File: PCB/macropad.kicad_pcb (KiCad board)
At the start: 2 copper layers, 4 parts, among them SW1 SW_Push, SW2 SW_Push, SW3 SW_Push, U1 MOUDLE-SEEEDUINO-XIAO

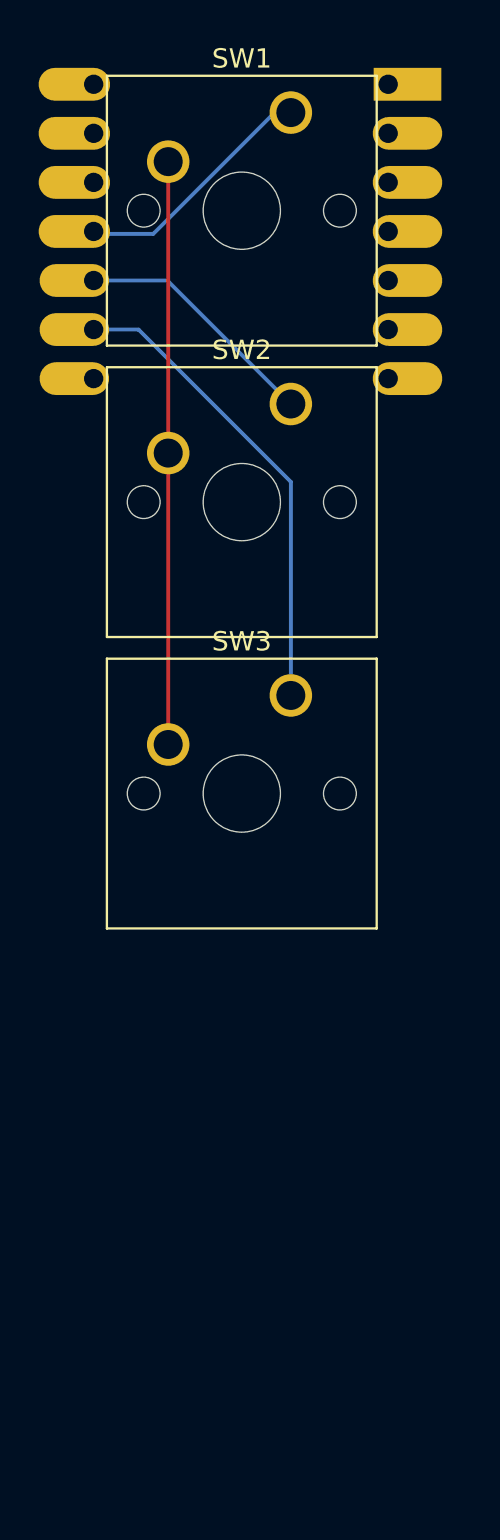
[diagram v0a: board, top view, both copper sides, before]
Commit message: Refactor code structure for improved readability and maintainability
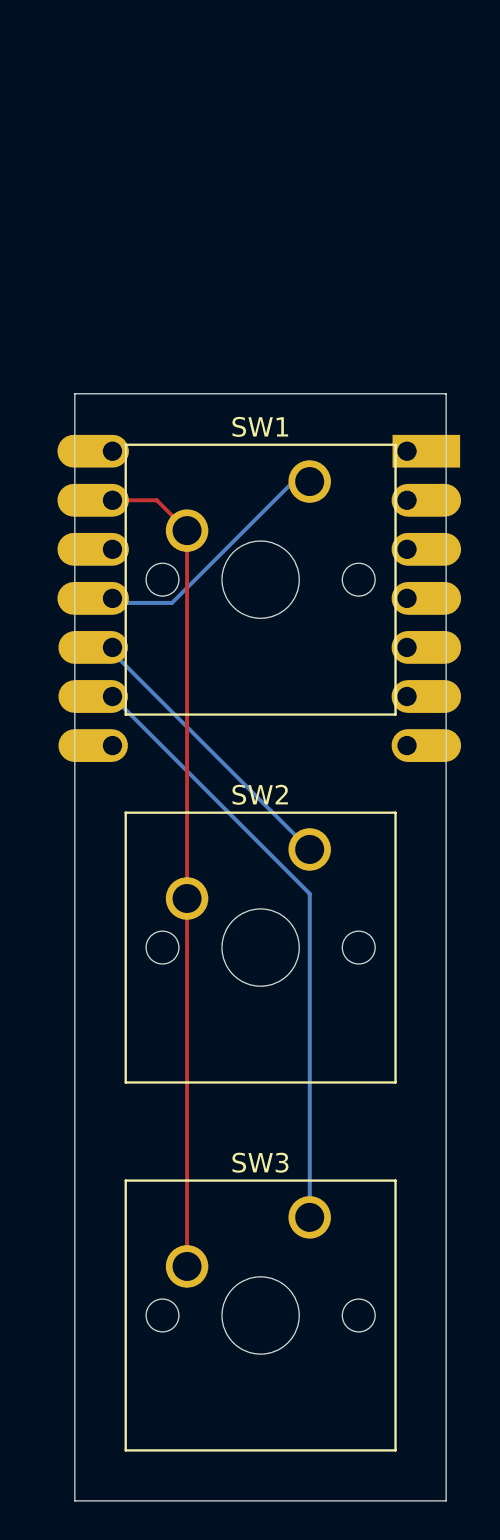
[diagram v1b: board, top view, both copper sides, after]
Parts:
- moved SW3 27.0 mm to (134.1, 119.2)
- moved SW2 23.1 mm to (134.1, 100.1)
- moved SW1 19.1 mm to (134.1, 81.1)
- moved U1 19.0 mm to (131.5, 87.1)
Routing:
- net GND: track 30.2 -> 42.7 mm
- net Net-(U1-PA7_A8_D8_SCK): track 24.5 -> 31.2 mm
- net Net-(U1-PA5_A9_D9_MISO): track 12.9 -> 14.7 mm
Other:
- board outline added: 19.2 x 57.3 mm
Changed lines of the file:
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@@
 	(footprint "Button_Switch_Keyboard:SW_Cherry_MX_1.00u_PCB"
 		(layer "F.Cu")
-		(at 133.085 61.965)
+		(at 134.06 81.07)
 		(descr "Cherry MX keyswitch, 1.00u, PCB mount, http://cherryamericas.com/wp-content/uploads/2014/12/mx_cat.pdf")
 		(tags "Cherry MX keyswitch 1.00u PCB")
@@
 	(footprint "Button_Switch_Keyboard:SW_Cherry_MX_1.00u_PCB"
 		(layer "F.Cu")
-		(at 133.085 77.055)
+		(at 134.06 100.12)
 		(descr "Cherry MX keyswitch, 1.00u, PCB mount, http://cherryamericas.com/wp-content/uploads/2014/12/mx_cat.pdf")
 		(tags "Cherry MX keyswitch 1.00u PCB")
@@
 	(footprint "Button_Switch_Keyboard:SW_Cherry_MX_1.00u_PCB"
 		(layer "F.Cu")
-		(at 133.085 92.145)
+		(at 134.06 119.17)
 		(descr "Cherry MX keyswitch, 1.00u, PCB mount, http://cherryamericas.com/wp-content/uploads/2014/12/mx_cat.pdf")
 		(tags "Cherry MX keyswitch 1.00u PCB")
@@
 	(footprint "footprints:XIAO-Generic-Hybrid-14P-2.54-21X17.8MM"
 		(layer "B.Cu")
-		(at 130.5 68.12 180)
+		(at 131.475 87.12 180)
 		(property "Reference" "U1"
 			(at 0 -2.54 0)
@@
 		(embedded_fonts no)
 	)
-	(segment
-		(start 126.735 94.685)
-		(end 126.735 79.595)
-		(width 0.2)
-		(layer "F.Cu")
-		(net "GND")
+	(gr_rect
+		(start 121.9 76.525)
+		(end 141.125 133.85)
+		(stroke
+			(width 0.05)
+			(type default)
+		)
+		(fill no)
+		(layer "Edge.Cuts")
 	)
 	(segment
-		(start 126.735 79.595)
-		(end 126.735 64.505)
+		(start 126.937056 87.35)
+		(end 124.08 87.35)
 		(width 0.2)
-		(layer "F.Cu")
-		(net "GND")
+		(layer "B.Cu")
+		(net "Net-(U1-PA6_A10_D10_MOSI)")
 	)
 	(segment
-		(start 125.962056 68.245)
-		(end 123 68.245)
+		(start 133.217056 81.07)
+		(end 126.937056 87.35)
 		(width 0.2)
 		(layer "B.Cu")
@@
 	)
 	(segment
-		(start 132.242056 61.965)
-		(end 125.962056 68.245)
+		(start 134.06 81.07)
+		(end 133.217056 81.07)
 		(width 0.2)
 		(layer "B.Cu")
@@
 	)
 	(segment
-		(start 133.085 61.965)
-		(end 132.242056 61.965)
+		(start 124.08 87.35)
+		(end 123.85 87.12)
 		(width 0.2)
 		(layer "B.Cu")
@@
 	)
 	(segment
-		(start 123 68.245)
-		(end 122.875 68.12)
+		(start 127.71 121.29)
+		(end 127.71 102.66)
 		(width 0.2)
-		(layer "B.Cu")
-		(net "Net-(U1-PA6_A10_D10_MOSI)")
+		(layer "F.Cu")
+		(net "GND")
 	)
 	(segment
-		(start 126.69 70.66)
-		(end 122.875 70.66)
+		(start 126.14 82.04)
+		(end 123.85 82.04)
 		(width 0.2)
-		(layer "B.Cu")
-		(net "Net-(U1-PA5_A9_D9_MISO)")
+		(layer "F.Cu")
+		(net "GND")
+	)
+	(segment
+		(start 127.6 121.4)
+		(end 127.71 121.29)
+		(width 0.2)
+		(layer "F.Cu")
+		(net "GND")
 	)
 	(segment
-		(start 133.085 77.055)
-		(end 126.69 70.66)
+		(start 127.71 102.66)
+		(end 127.71 83.61)
+		(width 0.2)
+		(layer "F.Cu")
+		(net "GND")
+	)
+	(segment
+		(start 127.71 121.71)
+		(end 127.71 121.51)
+		(width 0.2)
+		(layer "F.Cu")
+		(net "GND")
+	)
+	(segment
+		(start 127.71 121.51)
+		(end 127.6 121.4)
+		(width 0.2)
+		(layer "F.Cu")
+		(net "GND")
+	)
+	(segment
+		(start 127.71 83.61)
+		(end 126.14 82.04)
+		(width 0.2)
+		(layer "F.Cu")
+		(net "GND")
+	)
+	(segment
+		(start 134.06 100.12)
+		(end 123.85 89.91)
 		(width 0.2)
 		(layer "B.Cu")
@@
 	)
 	(segment
-		(start 125.2 73.2)
-		(end 122.875 73.2)
+		(start 123.85 89.91)
+		(end 123.85 89.66)
 		(width 0.2)
 		(layer "B.Cu")
-		(net "Net-(U1-PA7_A8_D8_SCK)")
+		(net "Net-(U1-PA5_A9_D9_MISO)")
 	)
 	(segment
-		(start 133.085 81.085)
-		(end 125.2 73.2)
+		(start 134.06 102.41)
+		(end 123.85 92.2)
 		(width 0.2)
 		(layer "B.Cu")
@@
 	)
 	(segment
-		(start 133.085 92.145)
-		(end 133.085 81.085)
+		(start 134.06 119.17)
+		(end 134.06 102.41)
 		(width 0.2)
 		(layer "B.Cu")
